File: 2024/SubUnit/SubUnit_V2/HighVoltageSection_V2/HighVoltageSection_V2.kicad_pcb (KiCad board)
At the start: 2 copper layers, 62.2 x 24.4 mm, 17 parts, among them J1 Conn_01x02_Socket, J10 Conn_01x02_Socket, J2 Conn_01x02_Socket, J3 Conn_01x02_Socket, J4 Conn_01x02_Socket, J6 Conn_01x02_Socket, J7 Conn_01x02_Socket, Q2 NMOS, Q3 NMOS

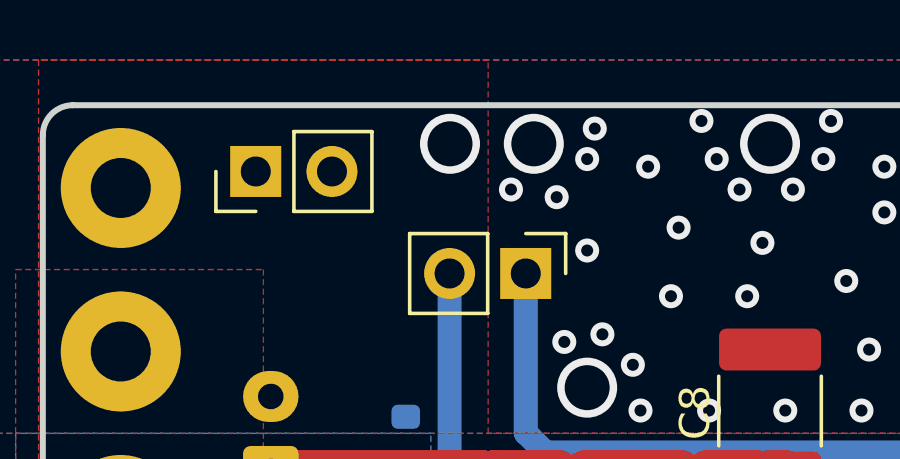
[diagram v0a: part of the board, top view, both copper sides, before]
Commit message: 完成
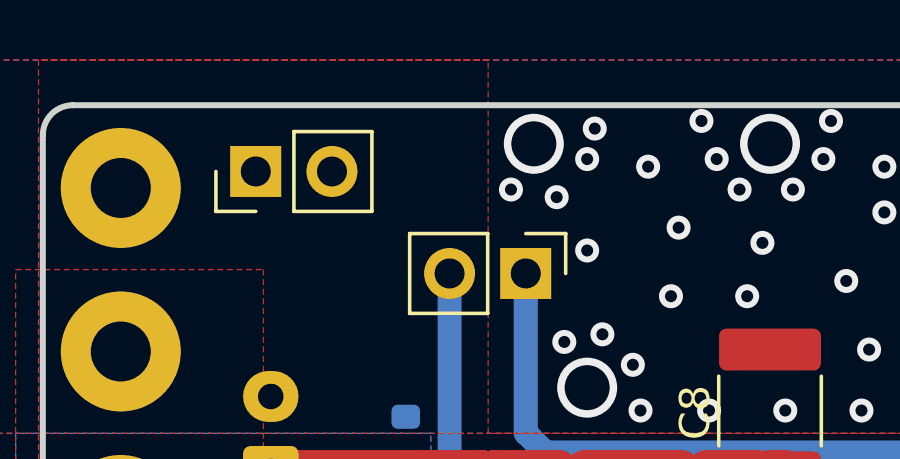
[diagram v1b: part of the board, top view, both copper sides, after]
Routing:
- net VOUT: vias 50 -> 49
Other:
- board text added: "CAPACITOR"
- board text added: "GND"
- board text added: "SOLENOID"
- board text added: "VOUT"
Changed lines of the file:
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@@
         (effects (font (size 1 1) (thickness 0.15)))
     )
-    (fp_text user "${REFERENCE}" (at 0 1.27) (layer "F.Fab")
-        (effects (font (size 1 1) (thickness 0.15)))
-    )
     (fp_line (start -1.33 -1.33) (end 0 -1.33)
       (stroke (width 0.12) (type solid)) (layer "F.SilkS"))
@@
     (property "ki_keywords" "R res resistor")
     (attr smd)
-    (fp_text reference "R9" (at 3 0 90) (layer "B.SilkS")
+    (fp_text reference "R9" (at 0.016 1.474 90) (layer "B.SilkS")
         (effects (font (size 1 1) (thickness 0.15)) (justify mirror))
     )
@@
         (effects (font (size 1 1) (thickness 0.1)) (justify mirror))
     )
-    (fp_text value "NMOS" (at 0 -1 90 unlocked) (layer "B.Fab")
+    (fp_text value "NMOS" (at 0 -1 90 unlocked) (layer "B.Fab") hide
         (effects (font (size 1 1) (thickness 0.15)) (justify mirror))
     )
@@
         (effects (font (size 1 1) (thickness 0.1)) (justify left bottom mirror))
     )
-    (fp_text user "${REFERENCE}" (at 0 -2.5 90 unlocked) (layer "B.Fab")
-        (effects (font (size 1 1) (thickness 0.15)) (justify mirror))
-    )
     (fp_text user "drain" (at -2 -5 90 unlocked) (layer "B.Fab")
         (effects (font (size 1 1) (thickness 0.1)) (justify left bottom mirror))
@@
         (effects (font (size 1 1) (thickness 0.15)) (justify mirror))
     )
-    (fp_text user "${REFERENCE}" (at 1.25 2.4 90) (layer "B.Fab")
-        (effects (font (size 1 1) (thickness 0.15)) (justify mirror))
-    )
     (fp_line (start -2.86 -2.21) (end -0.45 -2.21)
       (stroke (width 0.12) (type solid)) (layer "B.SilkS"))
@@
     (property "ki_keywords" "R res resistor")
     (attr smd)
-    (fp_text reference "R8" (at 0 1.5 90) (layer "B.SilkS")
+    (fp_text reference "R8" (at 0 -1.474 90) (layer "B.SilkS")
         (effects (font (size 1 1) (thickness 0.15)) (justify mirror))
     )
@@
     (property "ki_keywords" "diode TVS voltage suppressor")
     (attr smd)
-    (fp_text reference "D2" (at 0.038184 -2.119906 135) (layer "B.SilkS")
+    (fp_text reference "D2" (at -1.093187 2.046367 135) (layer "B.SilkS") hide
         (effects (font (size 1 1) (thickness 0.15)) (justify mirror))
     )
@@
     (property "ki_keywords" "R res resistor")
     (attr smd)
-    (fp_text reference "R10" (at 0 -1.25 -270) (layer "B.SilkS")
+    (fp_text reference "R10" (at 0.032 1.474 -270) (layer "B.SilkS")
         (effects (font (size 1 1) (thickness 0.15)) (justify mirror))
     )
@@
     (property "ki_keywords" "R res resistor")
     (attr smd)
-    (fp_text reference "R11" (at 3.25 0 -270) (layer "B.SilkS")
+    (fp_text reference "R11" (at 0.016 -1.474 -270) (layer "B.SilkS")
         (effects (font (size 1 1) (thickness 0.15)) (justify mirror))
     )
@@
   (gr_line locked (start -13.019294 2.790812) (end -0.000004 2.790812)
     (stroke (width 0.2) (type solid)) (layer "Edge.Cuts"))
+  (gr_text "SOLENOID" (at 17.399 6.35 -45) (layer "B.SilkS")
+    (effects (font (size 0.7 0.7) (thickness 0.14) bold italic) (justify left bottom mirror))
+  )
+  (gr_text "GND" (at 23.876 -7.62) (layer "B.SilkS")
+    (effects (font (size 0.7 0.7) (thickness 0.14) bold italic) (justify left bottom mirror))
+  )
+  (gr_text "CAPACITOR" (at -20.066 -5.588) (layer "B.SilkS")
+    (effects (font (size 0.7 0.7) (thickness 0.14) bold italic) (justify left bottom mirror))
+  )
+  (gr_text "CAPACITOR" (at 25.908 -5.588) (layer "B.SilkS")
+    (effects (font (size 0.7 0.7) (thickness 0.14) bold italic) (justify left bottom mirror))
+  )
+  (gr_text "VOUT" (at -21.336 -7.62) (layer "B.SilkS")
+    (effects (font (size 0.7 0.7) (thickness 0.14) bold italic) (justify left bottom mirror))
+  )
+  (gr_text "SOLENOID" (at -13.589 2.54 45) (layer "B.SilkS")
+    (effects (font (size 0.7 0.7) (thickness 0.14) bold italic) (justify left bottom mirror))
+  )
   (gr_text "BoostCircuitHighVoltageSection3.0\n20240505\nKotaroOCHIISHI" (at 0.254 -1.397) (layer "B.SilkS")
     (effects (font (size 0.7 0.7) (thickness 0.1) italic) (justify left bottom mirror))
@@
   (via (at -5.842 0.508) (size 0.8) (drill 0.4) (layers "F.Cu" "B.Cu") (net 2))
   (via (at -24.892 10.16) (size 0.8) (drill 0.4) (layers "F.Cu" "B.Cu") (free) (net 2))
-  (via (at -17.526 -10.922) (size 2) (drill 1.5) (layers "F.Cu" "B.Cu") (free) (net 2))
   (via (at 25.4 9.906) (size 0.8) (drill 0.4) (layers "F.Cu" "B.Cu") (free) (net 2))
   (via (at 23.368 11.684) (size 0.8) (drill 0.4) (layers "F.Cu" "B.Cu") (free) (net 2))
